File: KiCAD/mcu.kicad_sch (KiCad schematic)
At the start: 37 parts, among them SW69 RotaryEncoder_Switch, U69 W25Q32JVSS, U70 RP2040, U71 FM24CL16B, Y1 12MHz

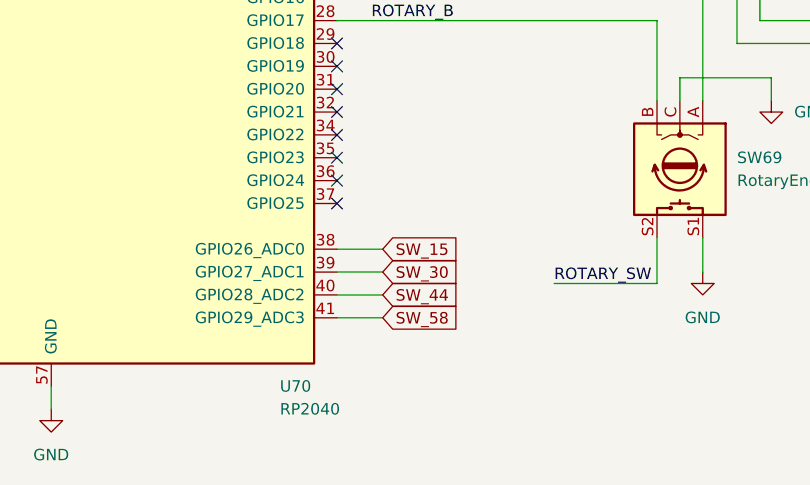
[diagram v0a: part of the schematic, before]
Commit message: Committing before changing to MUX design
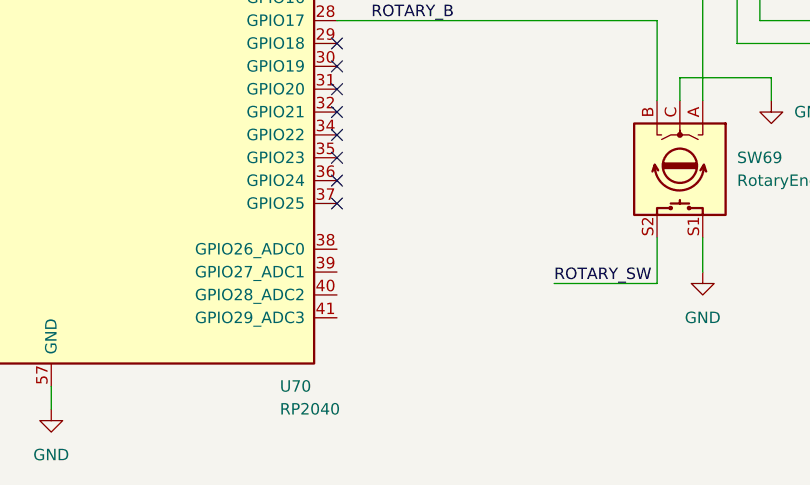
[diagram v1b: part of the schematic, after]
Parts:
- SW69: footprint (none) -> mini-general-tweaks:RotaryEncoder_Alps_EC11E-Switch-Vertical-EDIT
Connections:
- net SW_15: no longer names the net of U70.38 (GPIO26_ADC0)
- net SW_30: no longer names the net of U70.39 (GPIO27_ADC1)
- net SW_44: no longer names the net of U70.40 (GPIO28_ADC2)
- net SW_58: no longer names the net of U70.41 (GPIO29_ADC3)
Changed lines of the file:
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@@
-    (stroke (width 0) (type default) (color 0 0 0 0))
-  )
-  (wire (pts (xy 161.29 143.51) (xy 166.37 143.51))
     (stroke (width 0) (type default) (color 0 0 0 0))
   )
@@
     (stroke (width 0) (type default) (color 0 0 0 0))
   )
-  (wire (pts (xy 161.29 140.97) (xy 166.37 140.97))
-    (stroke (width 0) (type default) (color 0 0 0 0))
-  )
   (wire (pts (xy 109.22 26.67) (xy 109.22 27.94))
     (stroke (width 0) (type default) (color 0 0 0 0))
@@
     (stroke (width 0) (type default) (color 0 0 0 0))
   )
-  (wire (pts (xy 161.29 138.43) (xy 166.37 138.43))
-    (stroke (width 0) (type default) (color 0 0 0 0))
-  )
   (wire (pts (xy 179.07 96.52) (xy 187.96 96.52))
     (stroke (width 0) (type default) (color 0 0 0 0))
@@
   )
   (wire (pts (xy 27.94 77.47) (xy 27.94 78.74))
-    (stroke (width 0) (type default) (color 0 0 0 0))
-  )
-  (wire (pts (xy 161.29 146.05) (xy 166.37 146.05))
     (stroke (width 0) (type default) (color 0 0 0 0))
   )
@@
     )
   )
-  (global_label "SW_15" (shape input) (at 166.37 138.43 0) (fields_autoplaced)
-    (effects (font (size 1.27 1.27)) (justify left))
-    (property "Intersheet References" "${INTERSHEET_REFS}" (id 0) (at 174.8307 138.3506 0)
-      (effects (font (size 1.27 1.27)) (justify left) hide)
-    )
-  )
   (global_label "USB_D+" (shape input) (at 162.56 59.69 0) (fields_autoplaced)
     (effects (font (size 1.27 1.27)) (justify left))
@@
     )
   )
-  (global_label "SW_44" (shape input) (at 166.37 143.51 0) (fields_autoplaced)
-    (effects (font (size 1.27 1.27)) (justify left))
-    (property "Intersheet References" "${INTERSHEET_REFS}" (id 0) (at 174.8307 143.4306 0)
-      (effects (font (size 1.27 1.27)) (justify left) hide)
-    )
-  )
   (global_label "LED_SCL" (shape input) (at 191.77 107.95 0) (fields_autoplaced)
     (effects (font (size 1.27 1.27)) (justify left))
@@
     )
   )
-  (global_label "SW_30" (shape input) (at 166.37 140.97 0) (fields_autoplaced)
-    (effects (font (size 1.27 1.27)) (justify left))
-    (property "Intersheet References" "${INTERSHEET_REFS}" (id 0) (at 174.8307 140.8906 0)
-      (effects (font (size 1.27 1.27)) (justify left) hide)
-    )
-  )
   (global_label "SPI1_SCLK" (shape input) (at 238.76 85.09 0) (fields_autoplaced)
     (effects (font (size 1.27 1.27)) (justify left))
@@
     (effects (font (size 1.27 1.27)) (justify left))
     (property "Intersheet References" "${INTERSHEET_REFS}" (id 0) (at 251.0307 77.3906 0)
-      (effects (font (size 1.27 1.27)) (justify left) hide)
-    )
-  )
-  (global_label "SW_58" (shape input) (at 166.37 146.05 0) (fields_autoplaced)
-    (effects (font (size 1.27 1.27)) (justify left))
-    (property "Intersheet References" "${INTERSHEET_REFS}" (id 0) (at 174.8307 145.9706 0)
       (effects (font (size 1.27 1.27)) (justify left) hide)
     )
@@
       (effects (font (size 1.27 1.27)) (justify left))
     )
-    (property "Footprint" "" (id 2) (at 203.454 125.73 0)
-      (effects (font (size 1.27 1.27)) hide)
-    )
+    (property "Footprint" "mini-general-tweaks:RotaryEncoder_Alps_EC11E-Switch-Vertical-EDIT" (id 2) (at 203.454 125.73 0)
+      (effects (font (size 1.27 1.27)) hide)
+    )

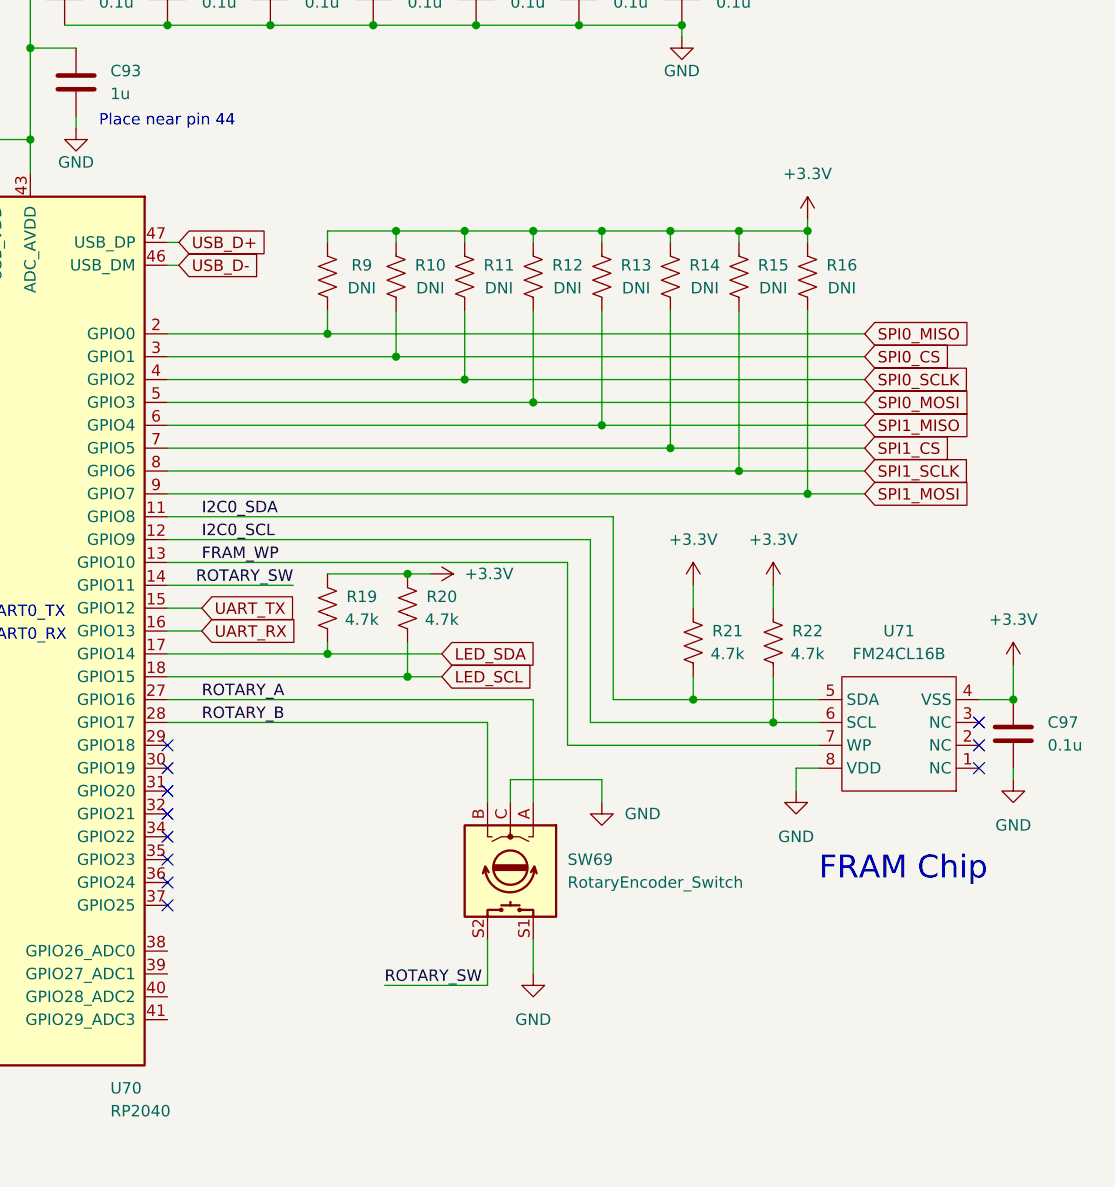
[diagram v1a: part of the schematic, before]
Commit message: Finished initial routing of PCB
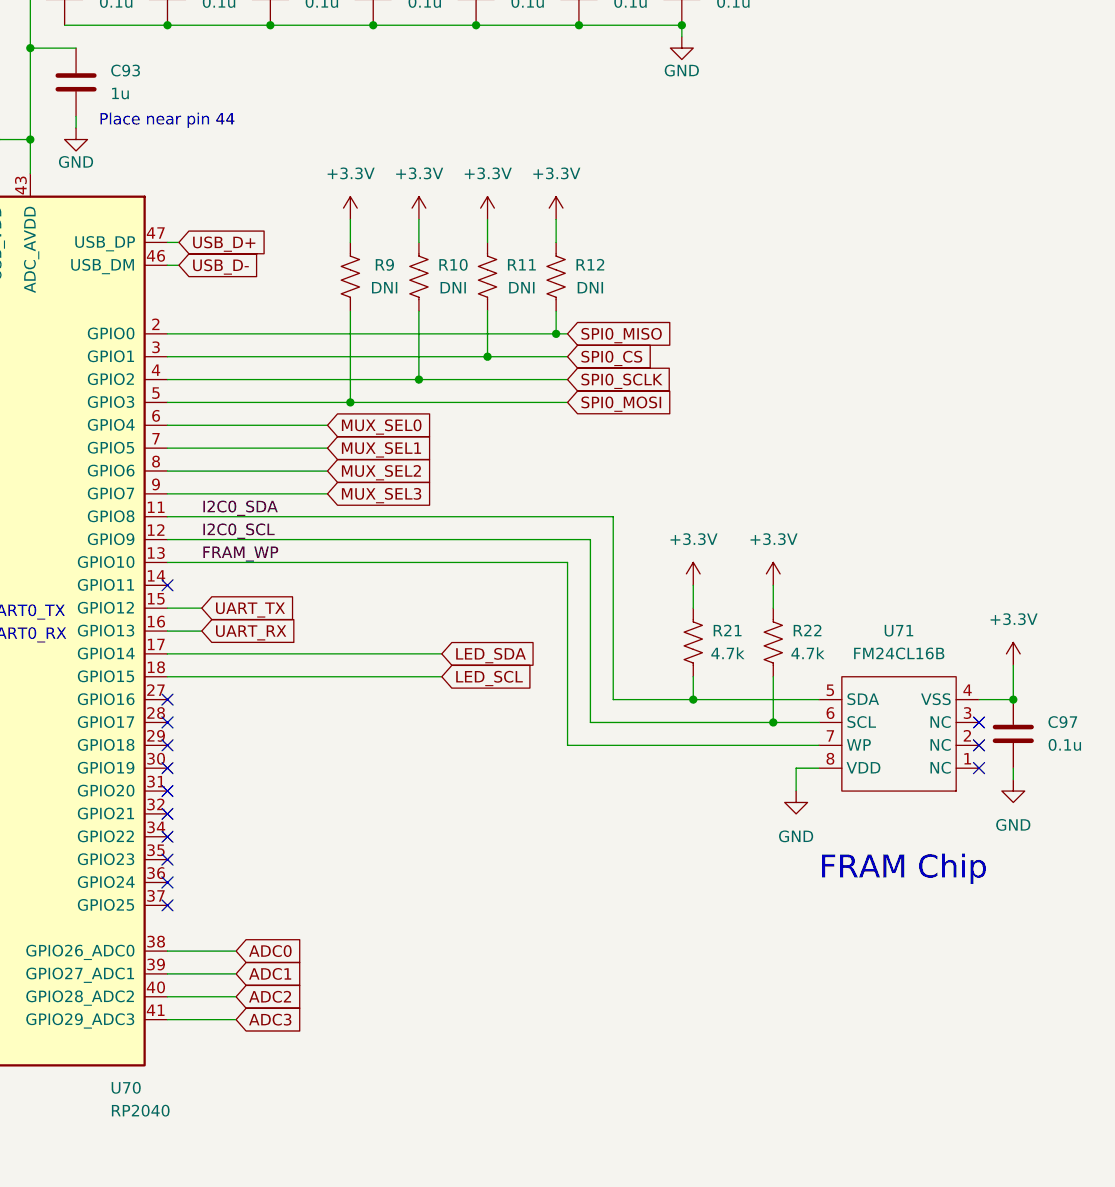
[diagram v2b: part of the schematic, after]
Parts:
- removed R13, R14, R15, R16: DNI, Resistor_SMD:R_0603_1608Metric_Pad0.98x0.95mm_HandSolder, symbol Device:R_US
- removed R19, R20: 4.7k, Resistor_SMD:R_0603_1608Metric_Pad0.98x0.95mm_HandSolder, symbol Device:R_US
- removed SW69: RotaryEncoder_Switch, mini-general-tweaks:RotaryEncoder_Alps_EC11E-Switch-Vertical-EDIT, symbol Device:RotaryEncoder_Switch
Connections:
- net SPI0_CS: now also R11.2; no longer R10.2
- net SPI0_MISO: now also R12.2; no longer R9.2
- net SPI0_MOSI: now also R9.2; no longer R12.2
- net SPI0_SCLK: now also R10.2; no longer R11.2
- net ADC0: now reaches U70.38 (GPIO26_ADC0)
- net ADC1: now reaches U70.39 (GPIO27_ADC1)
- net ADC2: now reaches U70.40 (GPIO28_ADC2)
- net ADC3: now reaches U70.41 (GPIO29_ADC3)
- net ROTARY_A: no longer names the net of U70.27 (GPIO16)
- net ROTARY_B: no longer names the net of U70.28 (GPIO17)
- net ROTARY_SW: no longer names the net of U70.14 (GPIO11)
- net SPI1_CS renamed MUX_SEL1
- net SPI1_MISO renamed MUX_SEL0
- net SPI1_MOSI renamed MUX_SEL3
- net SPI1_SCLK renamed MUX_SEL2
- no-connect marks 11 -> 14

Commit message: pushing various updates
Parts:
- R21, R22: Part Number (none) -> RMCF0603FT4K70
- U71: Part Number (none) -> FM24CL16B
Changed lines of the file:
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@@
+      (effects (font (size 1.27 1.27)) hide)
+    )
+    (property "Part Number" "FM24CL16B" (id 4) (at 242.57 118.11 0)
       (effects (font (size 1.27 1.27)) hide)
     )
@@
       (effects (font (size 1.27 1.27)) hide)
     )
+    (property "Part Number" "RMCF0603FT4K70" (id 4) (at 228.6 104.14 0)
+      (effects (font (size 1.27 1.27)) hide)
+    )
     (pin "1")
     (pin "2")
@@
       (effects (font (size 1.27 1.27)) hide)
     )
+    (property "Part Number" "RMCF0603FT4K70" (id 4) (at 219.71 104.14 0)
+      (effects (font (size 1.27 1.27)) hide)
+    )
